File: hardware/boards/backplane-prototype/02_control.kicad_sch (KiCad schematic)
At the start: 13 parts, among them J10 TC2030-IDC-NL SWD, U1 STM32C092GCU6

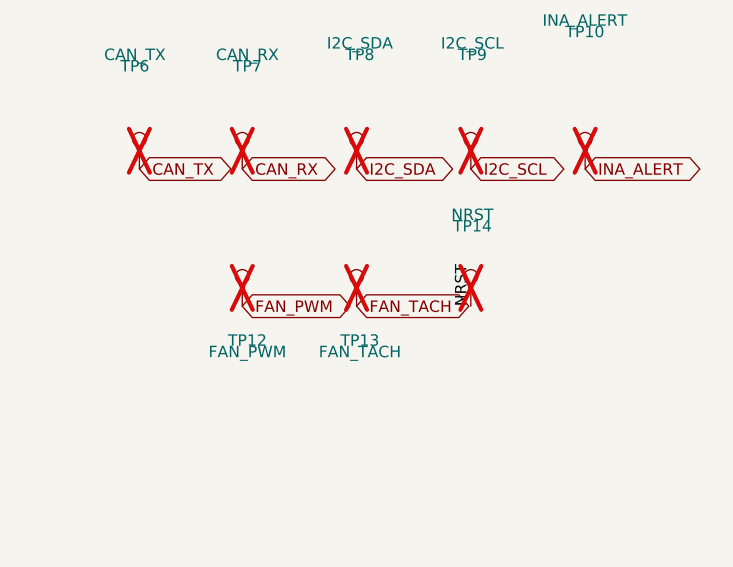
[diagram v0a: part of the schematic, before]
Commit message: checkpoint: save backplane layout updates
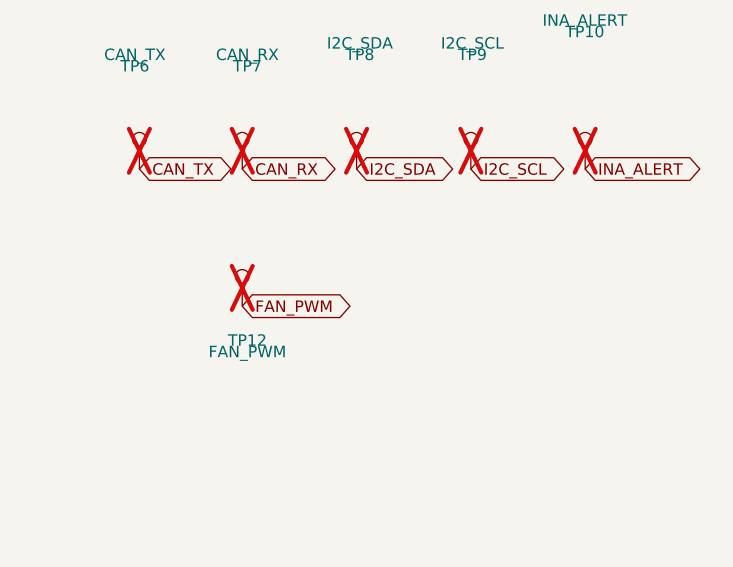
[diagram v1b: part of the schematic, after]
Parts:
- removed TP13: FAN_TACH, TestPoint:TestPoint_Pad_D1.5mm, symbol Connector:TestPoint
- removed TP14: NRST, TestPoint:TestPoint_Pad_D1.5mm, symbol Connector:TestPoint
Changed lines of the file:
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@@
 		(at 101.6 80.01)
-	)
-	(global_label "FAN2_PWM"
-		(shape bidirectional)
-		(at 137.16 87.63 0)
-		(effects
-			(font
-				(size 1.27 1.27)
-			)
-			(justify left)
-		)
-		(property "Intersheetrefs" "${INTERSHEET_REFS}"
-			(at 137.16 87.63 0)
-			(hide yes)
-			(show_name no)
-			(do_not_autoplace no)
-			(effects
-				(font
-					(size 1.27 1.27)
-				)
-			)
-		)
 	)
 	(no_connect
 		(at 137.16 82.55)
 	)
-	(global_label "FAN2_TACH"
-		(shape bidirectional)
-		(at 137.16 90.17 0)
-		(effects
-			(font
-				(size 1.27 1.27)
-			)
-			(justify left)
-		)
-		(property "Intersheetrefs" "${INTERSHEET_REFS}"
-			(at 137.16 90.17 0)
-			(hide yes)
-			(show_name no)
-			(do_not_autoplace no)
-			(effects
-				(font
-					(size 1.27 1.27)
-				)
-			)
-		)
-	)
 	(no_connect
 		(at 137.16 92.71)
@@
 		)
 	)
-	(global_label "DS18B20_DATA"
-		(shape bidirectional)
-		(at 101.6 105.41 180)
-		(effects
-			(font
-				(size 1.27 1.27)
-			)
-			(justify right)
-		)
-		(property "Intersheetrefs" "${INTERSHEET_REFS}"
-			(at 101.6 105.41 0)
-			(hide yes)
-			(show_name no)
-			(do_not_autoplace no)
-			(effects
-				(font
-					(size 1.27 1.27)
-				)
-			)
-		)
-	)
 	(label "SWCLK"
 		(at 67.31 115.57 180)
@@
 		)
 	)
-	(label "NRST"
-		(at 227.33 59.69 90)
-		(effects
-			(font
-				(size 1.27 1.27)
-			)
-			(justify left bottom)
-		)
-	)
 	(label "SWCLK"
 		(at 137.16 102.87 180)
@@
 		)
 	)
+	(global_label "DS18B20_DATA"
+		(shape bidirectional)
+		(at 101.6 105.41 180)
+		(effects
+			(font
+				(size 1.27 1.27)
+			)
+			(justify right)
+		)
+		(property "Intersheetrefs" "${INTERSHEET_REFS}"
+			(at 101.6 105.41 0)
+			(hide yes)
+			(show_name no)
+			(do_not_autoplace no)
+			(effects
+				(font
+					(size 1.27 1.27)
+				)
+			)
+		)
+	)
 	(global_label "+3V3"
 		(shape bidirectional)
@@
 		)
 	)
+	(global_label "FAN2_TACH"
+		(shape bidirectional)
+		(at 137.16 90.17 0)
+		(effects
+			(font
+				(size 1.27 1.27)
+			)
+			(justify left)
+		)
+		(property "Intersheetrefs" "${INTERSHEET_REFS}"
+			(at 137.16 90.17 0)
+			(hide yes)
+			(show_name no)
+			(do_not_autoplace no)
+			(effects
+				(font
+					(size 1.27 1.27)
+				)
+			)
+		)
+	)
 	(global_label "PGOOD_3V3"
 		(shape bidirectional)
@@
 		)
 	)
+	(global_label "FAN2_PWM"
+		(shape bidirectional)
+		(at 137.16 87.63 0)
+		(effects
+			(font
+				(size 1.27 1.27)
+			)
+			(justify left)
+		)
+		(property "Intersheetrefs" "${INTERSHEET_REFS}"
+			(at 137.16 87.63 0)
+			(hide yes)
+			(show_name no)
+			(do_not_autoplace no)
+			(effects
+				(font
+					(size 1.27 1.27)
+				)
+			)
+		)
+	)
 	(global_label "I2C_SDA"
 		(shape bidirectional)
@@
 		(property "Intersheetrefs" "${INTERSHEET_REFS}"
 			(at 64.77 48.26 0)
-			(hide yes)
-			(show_name no)
-			(do_not_autoplace no)
-			(effects
-				(font
-					(size 1.27 1.27)
-				)
-			)
-		)
-	)
-	(global_label "FAN_TACH"
-		(shape bidirectional)
-		(at 214.63 59.69 0)
-		(effects
-			(font
-				(size 1.27 1.27)
-			)
-			(justify left)
-		)
-		(property "Intersheetrefs" "${INTERSHEET_REFS}"
-			(at 214.63 59.69 0)
 			(hide yes)
 			(show_name no)
@@
 	(symbol
 		(lib_id "Connector:TestPoint")
-		(at 214.63 59.69 0)
-		(unit 1)
-		(body_style 1)
-		(exclude_from_sim no)
-		(in_bom no)
-		(on_board yes)
-		(in_pos_files yes)
-		(dnp yes)
-		(property "Reference" "TP13"
-			(at 215 63.5 0)
-			(show_name no)
-			(do_not_autoplace no)
-			(effects
-				(font
-					(size 1.27 1.27)
-				)
-			)
-		)
-		(property "Value" "FAN_TACH"
-			(at 215 64.77 0)
-			(show_name no)
-			(do_not_autoplace no)
-			(effects
-				(font
-					(size 1.27 1.27)
-				)
-			)
-		)
-		(property "Footprint" "TestPoint:TestPoint_Pad_D1.5mm"
-			(at 220.08 60 0)
-			(hide yes)
-			(show_name no)
-			(do_not_autoplace no)
-			(effects
-				(font
-					(size 1.27 1.27)
-				)
-			)
-		)
-		(property "Datasheet" ""
-			(at 220.08 60 0)
-			(hide yes)
-			(show_name no)
-			(do_not_autoplace no)
-			(effects
-				(font
-					(size 1.27 1.27)
-				)
-			)
-		)
-		(property "Description" "test point"
-			(at 215 60 0)
-			(hide yes)
-			(show_name no)
-			(do_not_autoplace no)
-			(effects
-				(font
-					(size 1.27 1.27)
-				)
-			)
-		)
-		(pin "1"
-		)
-		(instances
-			(project "backplane-prototype"
-				(path "/348cc909-6345-4013-9bef-98714057a65b/4275522b-7aaa-4a22-8d94-d30e15c87e30"
-					(reference "TP13")
-					(unit 1)
-				)
-			)
-		)
-	)
-	(symbol
-		(lib_id "Connector:TestPoint")
 		(at 201.93 59.69 0)
 		(unit 1)
@@
 					(unit 1)
 				)
-			)
-		)
-	)
-	(symbol
-		(lib_id "Connector:TestPoint")
-		(at 227.33 59.69 0)
-		(unit 1)
-		(body_style 1)
-		(exclude_from_sim no)
-		(in_bom no)
-		(on_board yes)
-		(in_pos_files yes)
-		(dnp yes)
-		(property "Reference" "TP14"
-			(at 227.5 50.8 0)
-			(show_name no)
-			(do_not_autoplace no)
-			(effects
-				(font
-					(size 1.27 1.27)
-				)
-			)
-		)
-		(property "Value" "NRST"
-			(at 227.5 49.53 0)
-			(show_name no)
-			(do_not_autoplace no)
-			(effects
-				(font
-					(size 1.27 1.27)
-				)
-			)
-		)
-		(property "Footprint" "TestPoint:TestPoint_Pad_D1.5mm"
-			(at 232.58 60 0)
-			(hide yes)
-			(show_name no)
-			(do_not_autoplace no)
-			(effects
-				(font
-					(size 1.27 1.27)
-				)
-			)
-		)
-		(property "Datasheet" ""
-			(at 232.58 60 0)
-			(hide yes)
-			(show_name no)
-			(do_not_autoplace no)
-			(effects
-				(font
-					(size 1.27 1.27)
-				)
-			)
-		)
-		(property "Description" "test point"
-			(at 227.5 60 0)
-			(hide yes)
-			(show_name no)
-			(do_not_autoplace no)
-			(effects
-				(font
-					(size 1.27 1.27)
-				)
-			)
-		)
-		(pin "1"
-		)
-		(instances
-			(project "backplane-prototype"
-				(path "/348cc909-6345-4013-9bef-98714057a65b/4275522b-7aaa-4a22-8d94-d30e15c87e30"
-					(reference "TP14")
-					(unit 1)
-				)
